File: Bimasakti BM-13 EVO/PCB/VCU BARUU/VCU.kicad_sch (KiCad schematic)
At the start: 8 parts, among them J1 6437288-3, J2 12V, J3 3V3_1, J4 3V3_2, J5 5V_1, J6 5V_2, J7 5V_3, J8 Conn_02x06_Top_Bottom

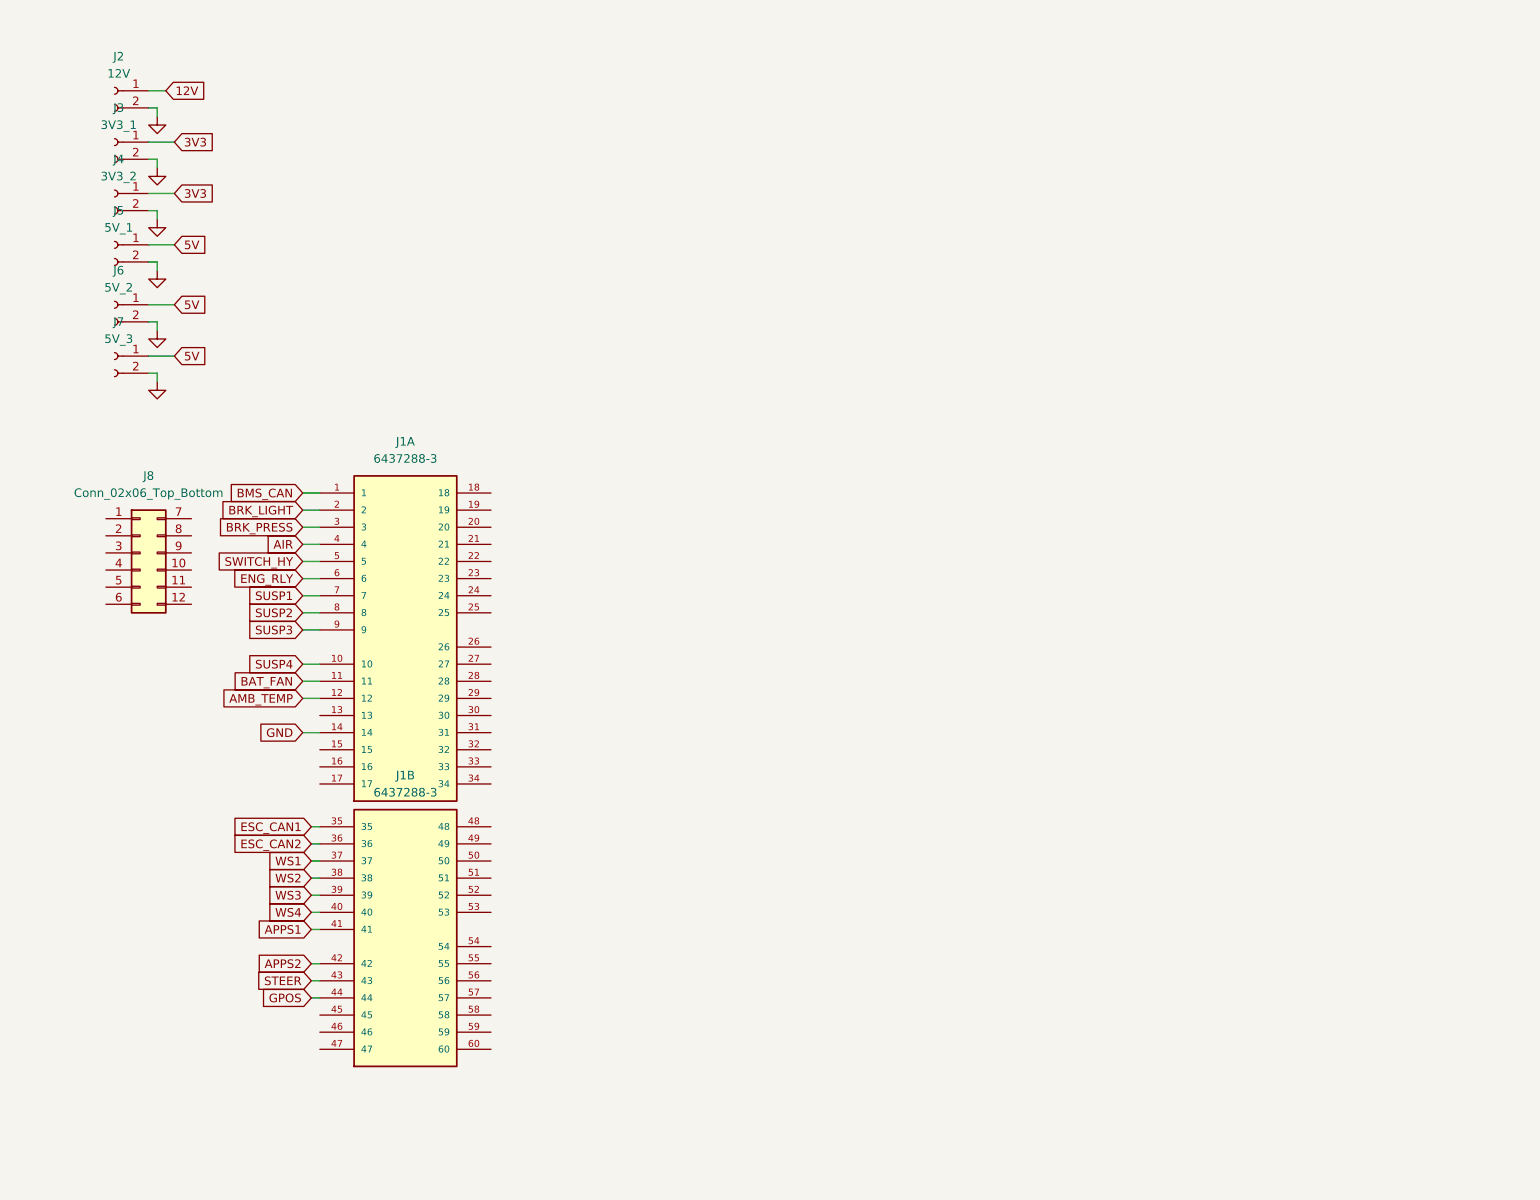
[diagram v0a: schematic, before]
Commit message: assembly kurang pneumatic, kurang wiring dudukan motherboard
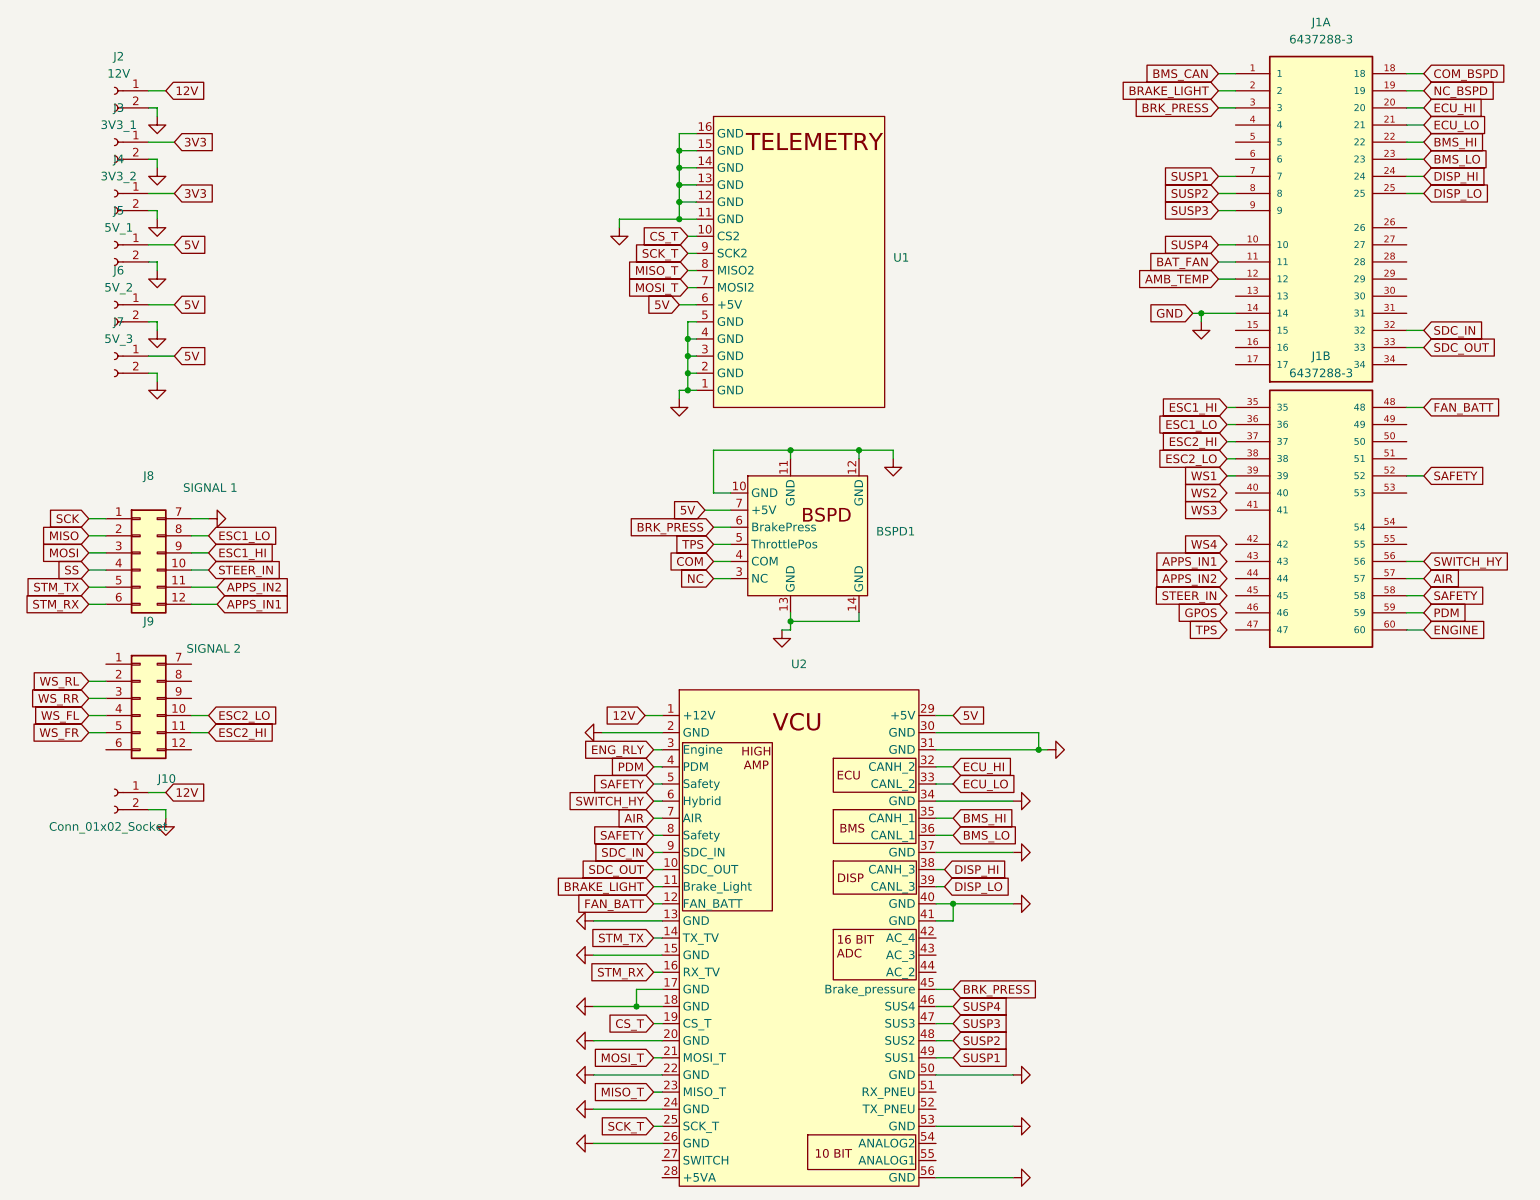
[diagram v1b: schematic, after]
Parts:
- added BSPD1: ~, 0_FootPrintBPSD:FootPrintBPSD, symbol 0_BSPDFootprint:FootprintBSPD
- added J10: Conn_01x02_Socket, Connector_Molex:Molex_Nano-Fit_105309-xx02_1x02_P2.50mm_Vertical, symbol Connector:Conn_01x02_Socket
- added J9: SIGNAL 2, Connector_Molex:Molex_Nano-Fit_105310-xx12_2x06_P2.50mm_Vertical, symbol Connector_Generic:Conn_02x06_Top_Bottom
- added U1: ~, 0_FootprintTelemetry:0_FootprintTelemetry, symbol 0_FootprintTelemetry:FootprintTelemetry
- added U2: ~, 0_FootprintVCU:FootprintVCU, symbol 0_FootprintVCU:FootprintVCU
- J8: value Conn_02x06_Top_Bottom -> SIGNAL 1
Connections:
- net ESC_CAN1 is gone; now on net ESC1_HI: J1.35
- net ESC_CAN2 is gone; now on net ESC1_LO: J1.36
- net 12V: now also J10.1 (Pin_1), U2.1 (+12V)
- net 5V: now also BSPD1.7 (+5V), U1.6 (+5V), U2.29 (+5V)
- net AIR: now also J1.57, U2.7 (AIR); no longer J1.4
- net BRK_PRESS: now also BSPD1.6 (BrakePress), U2.45 (Brake_pressure)
- net ENG_RLY: now also U2.3 (Engine); no longer J1.6
- net GND: now also J8.7 (Pin_7), BSPD1.10 (GND), BSPD1.11 (GND), BSPD1.12 (GND), BSPD1.13 (GND), BSPD1.14 (GND), J10.2 (Pin_2), U1.1 (GND), U1.11 (GND), U1.12 (GND), U1.13 (GND), U1.14 (GND), U1.15 (GND), U1.16 (GND), U1.2 (GND), U1.3 (GND), U1.4 (GND), U1.5 (GND), U2.13 (GND), U2.15 (GND), U2.17 (GND), U2.18 (GND), U2.2 (GND), U2.20 (GND), U2.22 (GND), U2.24 (GND), U2.26 (GND), U2.30 (GND), U2.31 (GND), U2.34 (GND), U2.37 (GND), U2.40 (GND), U2.41 (GND), U2.50 (GND), U2.53 (GND), U2.56 (GND)
- net GPOS: no longer J1.44
- net SUSP1: now also U2.49 (SUS1)
- net SUSP2: now also U2.48 (SUS2)
- net SUSP3: now also U2.47 (SUS3)
- net SUSP4: now also U2.46 (SUS4)
- net SWITCH_HY: now also J1.56, U2.6 (Hybrid); no longer J1.5
- net WS1: now also J1.39; no longer J1.37
- net WS2: no longer J1.38
- net WS3: no longer J1.39
- net WS4: no longer J1.40
- net SCK: now reaches J8.1 (Pin_1)
- net STEER_IN: now reaches J8.10 (Pin_10)
- net APPS_IN2: now reaches J8.11 (Pin_11)
- net APPS_IN1: now reaches J8.12 (Pin_12)
- net MISO: now reaches J8.2 (Pin_2)
- net MOSI: now reaches J8.3 (Pin_3)
- net SS: now reaches J8.4 (Pin_4)
- net STM_TX: now reaches J8.5 (Pin_5)
- net STM_TX: now also U2.14 (TX_TV)
- net STM_RX: now reaches J8.6 (Pin_6)
- net STM_RX: now also U2.16 (RX_TV)
- net ESC1_LO: now reaches J8.8 (Pin_8)
- net ESC1_HI: now reaches J8.9 (Pin_9)
- net COM_BSPD: now reaches J1.18
- net NC_BSPD: now reaches J1.19
- net ECU_HI: now reaches J1.20
- net ECU_HI: now also U2.32 (CANH_2)
- net ECU_LO: now reaches J1.21
- net ECU_LO: now also U2.33 (CANL_2)
- net BMS_HI: now reaches J1.22
- net BMS_HI: now also U2.35 (CANH_1)
- net BMS_LO: now reaches J1.23
- net BMS_LO: now also U2.36 (CANL_1)
- net DISP_HI: now reaches J1.24
- net DISP_HI: now also U2.38 (CANH_3)
- net DISP_LO: now reaches J1.25
- net DISP_LO: now also U2.39 (CANL_3)
- net SDC_IN: now reaches J1.32
- net SDC_IN: now also U2.9 (SDC_IN)
- net SDC_OUT: now reaches J1.33
- net SDC_OUT: now also U2.10 (SDC_OUT)
- net FAN_BATT: now reaches J1.48
- net FAN_BATT: now also U2.12 (FAN_BATT)
- net SAFETY: now reaches J1.52
- net SAFETY: now also J1.58, U2.5 (Safety), U2.8 (Safety)
- net PDM: now reaches J1.59
- net PDM: now also U2.4 (PDM)
- net ENGINE: now reaches J1.60
- net APPS1: no longer names the net of J1.41
- net APPS2: no longer names the net of J1.42
- net BRK_LIGHT renamed BRAKE_LIGHT
- net BRAKE_LIGHT: now also U2.11 (Brake_Light)
- net STEER: no longer names the net of J1.43
- new net COM: BSPD1.4 (COM)
- new net CS_T: U1.10 (CS2), U2.19 (CS_T)
- new net ESC2_HI: J1.37, J9.11 (Pin_11)
- new net ESC2_LO: J1.38, J9.10 (Pin_10)
- new net MISO_T: U1.8 (MISO2), U2.23 (MISO_T)
- new net MOSI_T: U1.7 (MOSI2), U2.21 (MOSI_T)
- new net NC: BSPD1.3 (NC)
- new net SCK_T: U1.9 (SCK2), U2.25 (SCK_T)
- new net TPS: BSPD1.5 (ThrottlePos)
- new net WS_FL: J9.4 (Pin_4)
- new net WS_FR: J9.5 (Pin_5)
- new net WS_RL: J9.2 (Pin_2)
- new net WS_RR: J9.3 (Pin_3)
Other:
- moved on the sheet: J1A, J1B
